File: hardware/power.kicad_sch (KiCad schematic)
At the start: 29 parts, among them J18 Line, J19 Neutral, J20 Earth, T1 3FD-516, U1 LM2575-5.0BT

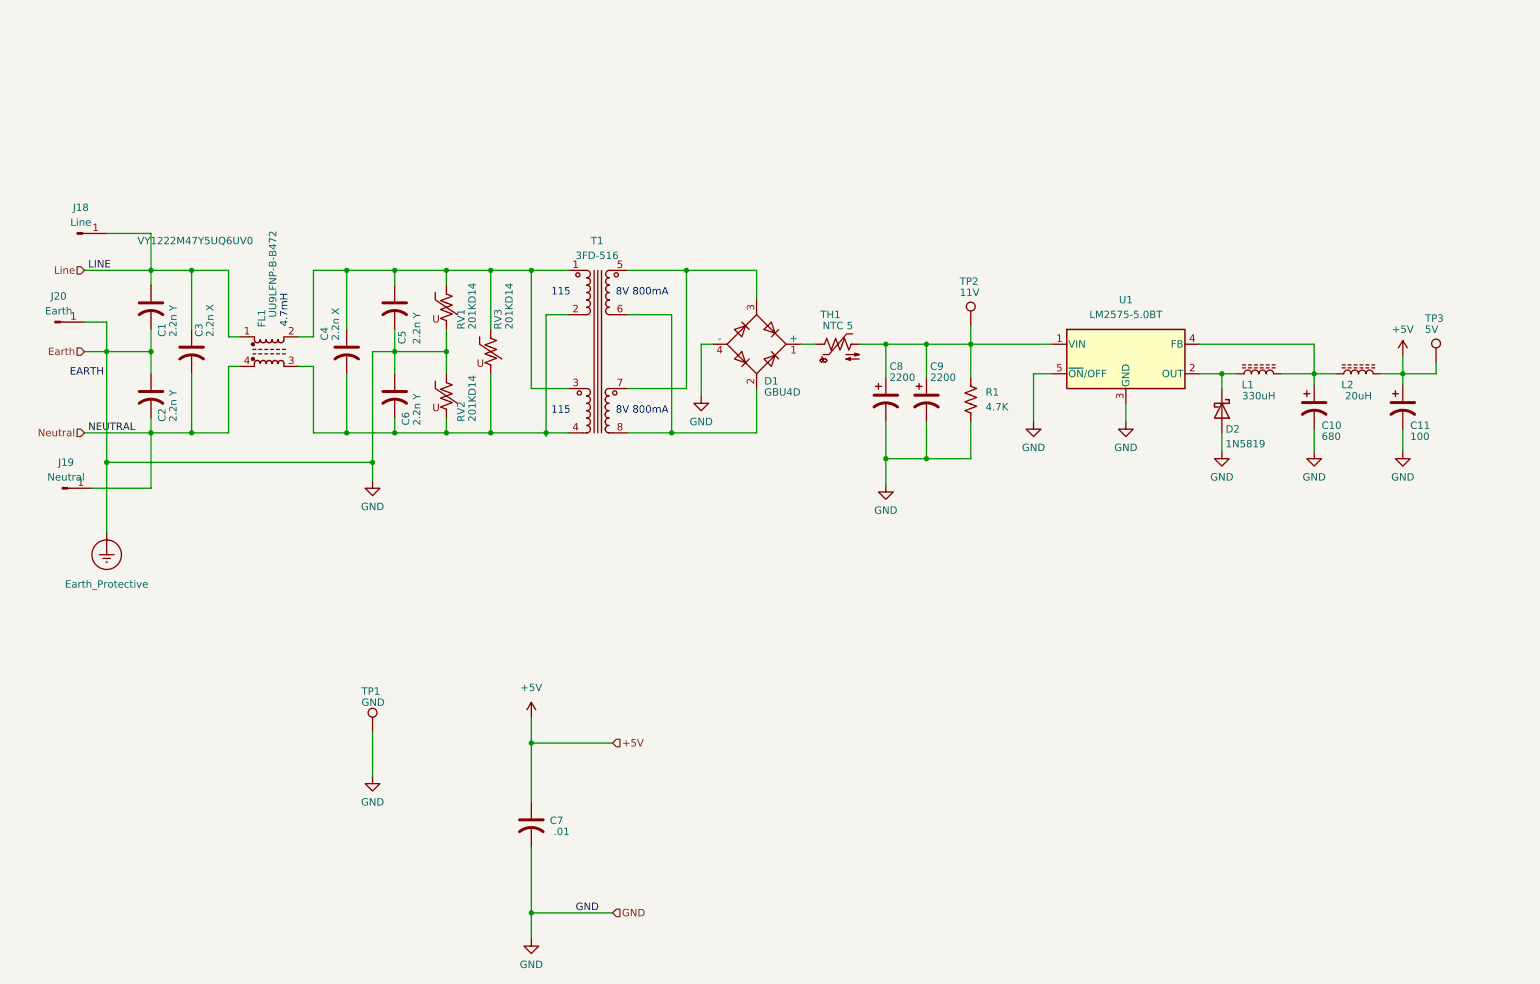
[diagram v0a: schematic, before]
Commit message: Revised hardware design
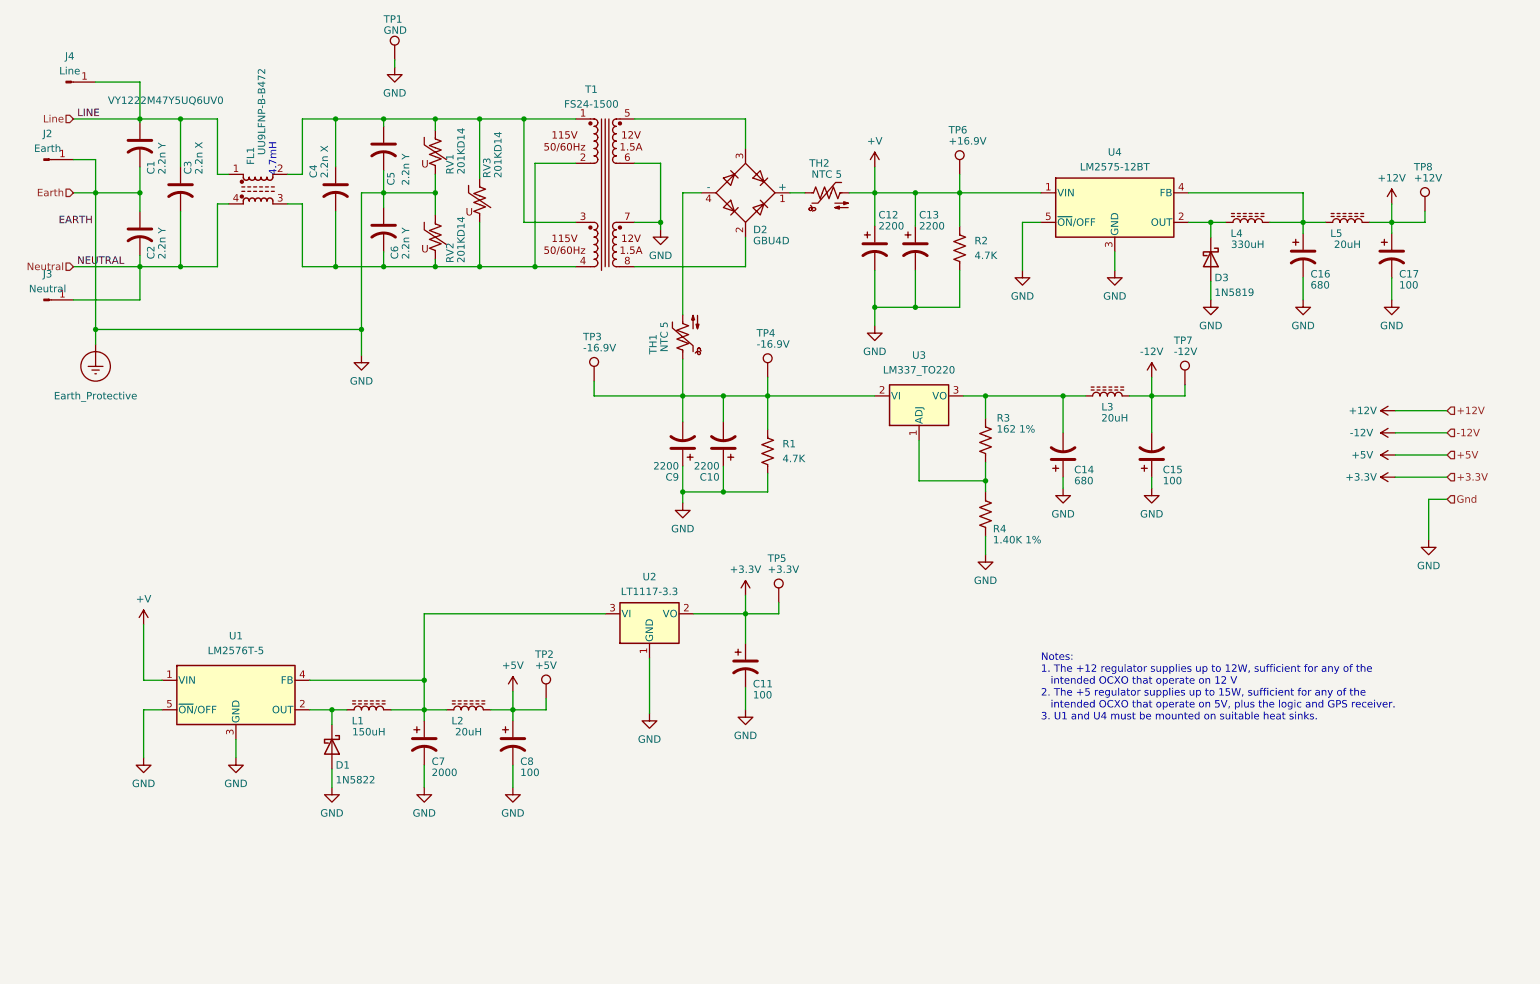
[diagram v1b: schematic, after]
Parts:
- removed C7: .01, Capacitor_SMD:C_0805_2012Metric_Pad1.18x1.45mm_HandSolder, symbol Device:C_US
- removed T1: 3FD-516, Transformers_Tamura:3FD, symbol Transformers_Tamura:3FD-516
- added C10, C9: 2200, Capacitor_THT:CP_Radial_D18.0mm_P7.50mm, symbol Device:C_Polarized_US
- added C11, C15, C8: 100, Capacitor_SMD:CP_Elec_6.3x7.7, symbol Device:C_Polarized_US
- added C14: 680, Capacitor_SMD:CP_Elec_10x10, symbol Device:C_Polarized_US
- added C7: 2000, Capacitor_SMD:CP_Elec_10x10, symbol Device:C_Polarized_US
- added D1: 1N5822, Diode_SMD:D_SOD-123, symbol Diode:1N5819
- added L1: 150uH, Inductor_SMD:L_12x12mm_H8mm, symbol Device:L_Ferrite
- added L2, L3: 20uH, Inductor_SMD:L_TDK_VLF10040, symbol Device:L_Ferrite
- added R1: 4.7K, Resistor_SMD:R_0805_2012Metric_Pad1.20x1.40mm_HandSolder, symbol Device:R_US
- added R3: 162 1%, Resistor_SMD:R_0805_2012Metric_Pad1.20x1.40mm_HandSolder, symbol Device:R_US
- added R4: 1.40K 1%, Resistor_SMD:R_0805_2012Metric_Pad1.20x1.40mm_HandSolder, symbol Device:R_US
- added T1: FS24-1500, Transformers_Triad:FS-36VA, symbol fs24-1500:FS24-1500
- added TH1: NTC 5, Capacitor_THT:C_Disc_D8.0mm_W5.0mm_P5.00mm, symbol Device:Thermistor_NTC_US
- added TP2: +5V, TestPoint:TestPoint_Bridge_Pitch2.54mm_Drill0.7mm, symbol Connector:TestPoint
- added TP3, TP4: -16.9V, TestPoint:TestPoint_Bridge_Pitch2.54mm_Drill0.7mm, symbol Connector:TestPoint
- added TP5: +3.3V, TestPoint:TestPoint_Bridge_Pitch2.54mm_Drill0.7mm, symbol Connector:TestPoint
- added TP7: -12V, TestPoint:TestPoint_Bridge_Pitch2.54mm_Drill0.7mm, symbol Connector:TestPoint
- added U1: LM2576T-5, Package_TO_SOT_THT:TO-220-5_Vertical, symbol Regulator_Switching:LM2576T-5
- added U2: LT1117-3.3, symbol Regulator_Linear:LT1117-3.3
- added U3: LM337_TO220, Package_TO_SOT_THT:TO-220-3_Vertical, symbol Regulator_Linear:LM337_TO220
- TP6: renamed from TP2; value 11V -> +16.9V
- TP8: renamed from TP3; value 5V -> +12V
- U4: renamed from U1; value LM2575-5.0BT -> LM2575-12BT
- renumbered C8 to C12, C9 to C13, C10 to C16, C11 to C17, D1 to D2, D2 to D3, J20 to J2, J19 to J3, J18 to J4, L1 to L4, L2 to L5, R1 to R2, TH1 to TH2
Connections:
- net +5V: now also C8.1, L2.2, TP2.1; no longer C17.1, L5.2, TP8.1
- net Earth_Protective: now also C10.1, C11.2, C14.1, C15.1, C7.2, C8.2, C9.1, D1.2 (A), R1.2, R4.2, T1.6, T1.7, U1.3 (GND), U1.5 (~{ON}/OFF), U2.1 (GND); no longer D2.4 (-)
- net +V: now reaches C12.1, C13.1, R2.1, TH2.2, TP6.1, U4.1 (VIN)
- net +V: now also U1.1 (VIN)
- net at C4.2, C6.2, FL1.3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: now also T1.2, T1.4
- net at C4.1, C5.1, FL1.2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: now also T1.1, T1.3
- net at D2.3: now also T1.5
- net at D2.2: now also T1.8
- new net: R3.2, R4.1, U3.1 (ADJ)
- new net: C10.2, C9.2, R1.1, TH1.1, TP3.1, TP4.1, U3.2 (VI)
- new net: C14.2, L3.1, R3.1, U3.3 (VO)
- new net: C7.1, L1.2, L2.1, U1.4 (FB), U2.3 (VI)
- new net: D2.4 (-), TH1.2
- new net: D1.1 (K), L1.1, U1.2 (OUT)
- new net +12V: C17.1, L5.2, TP8.1
- new net +3.3V: C11.1, TP5.1, U2.2 (VO)
- new net -12V: C15.2, L3.2, TP7.1
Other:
- note added: "Notes: 1. The +12 regulator supplies up to 12W, sufficient for any of the intended OCXO that operate on 12 V 2. The +5 regulator supplies up to 15W, sufficient for any of the intended OCXO that operate on 5V, plus the logic and GPS receiver. 3. U1 and U4 must be mounted on suitable heat sinks."
- note removed: "115"
- note removed: "8V 800mA"
- moved on the sheet: C1, C12, C13, C16, C17, C2, C3, C4, C5, C6, D2, D3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
